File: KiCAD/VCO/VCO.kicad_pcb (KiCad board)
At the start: 2 copper layers, 50 x 100 mm, 41 parts, among them J1 CV IN 1, J2 CV IN 2, J3 PWM, J4 SAW OUT, J5 PULSE OUT, J6 Conn_01x03_Pin, J7 Conn_01x03_Pin, Q1 NPN, T1 PNP, T2 NPN, U1 4069

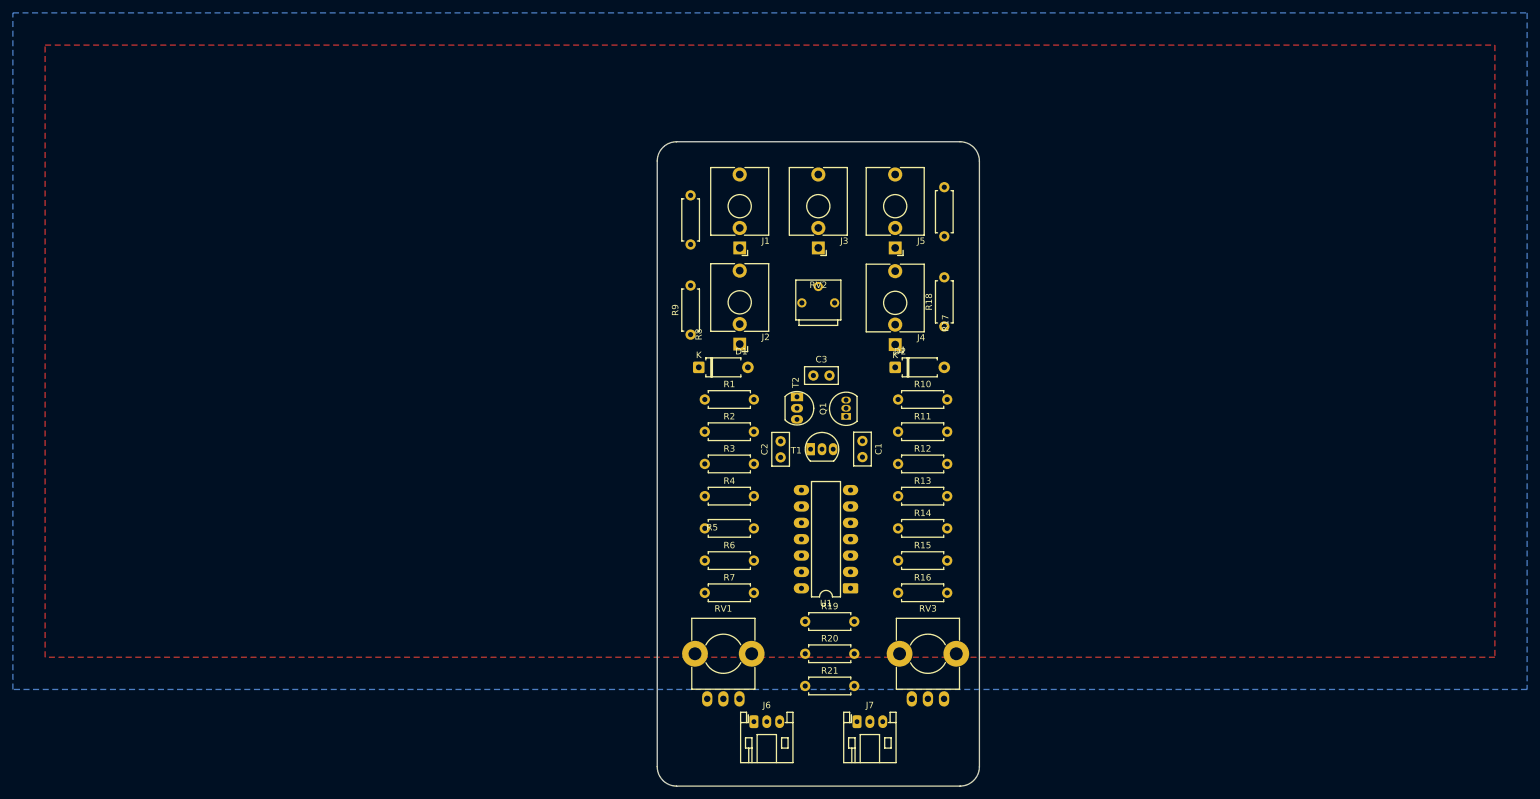
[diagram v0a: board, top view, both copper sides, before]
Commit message: Reapply VCO pcb layout changes.
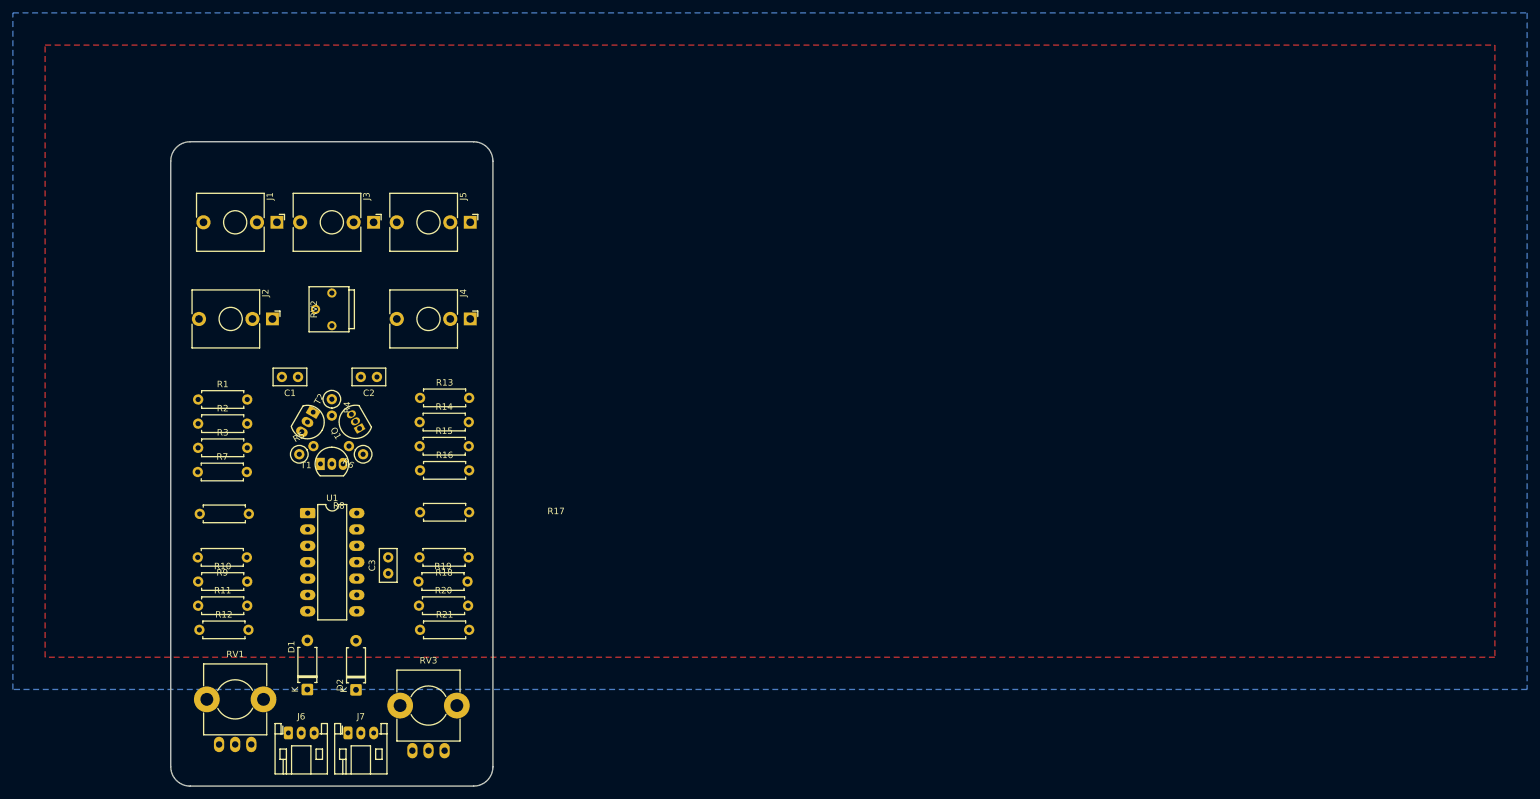
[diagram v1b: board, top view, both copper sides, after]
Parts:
- R4, R5, R6: footprint Resistor_THT:R_Axial_DIN0207_L6.3mm_D2.5mm_P7.62mm_Horizontal -> Resistor_THT:R_Axial_DIN0207_L6.3mm_D2.5mm_P2.54mm_Vertical
- moved R10 112.2 mm to (53.8, 118.2)
- moved R11 111.9 mm to (53.8, 122.0)
- moved R12 111.5 mm to (53.9, 125.8)
- moved D2 97.5 mm to (78.2, 135.1), turned to 90 degrees
- moved C1 88.2 mm to (69.2, 86.5), turned to 180 degrees
- moved R17 85.3 mm to (95.8, 107.5), turned to 180 degrees
- moved U1 85.1 mm to (70.8, 107.6), turned to 0 degrees
- moved R18 82.1 mm to (95.7, 114.5), turned to 180 degrees
- moved R7 80.9 mm to (53.7, 101.2)
- moved R8 80.3 mm to (61.6, 107.8), turned to 180 degrees
- moved J2 79.0 mm to (58.8, 77.5), turned to 90 degrees
- moved J7 79.0 mm to (77.0, 141.8)
- moved D1 78.7 mm to (70.7, 135.0), turned to 90 degrees
- moved R3 78.7 mm to (53.8, 97.5)
- moved R2 78.6 mm to (53.8, 93.8)
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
